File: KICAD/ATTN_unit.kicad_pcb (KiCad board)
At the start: 2 copper layers, 145.5 x 73.5 mm, 5 parts, among them SW1 SW_Push, U1 DM-OLED096-636, U2 HLK-LD2410C, U4 ESP32-DEVKITC-32E

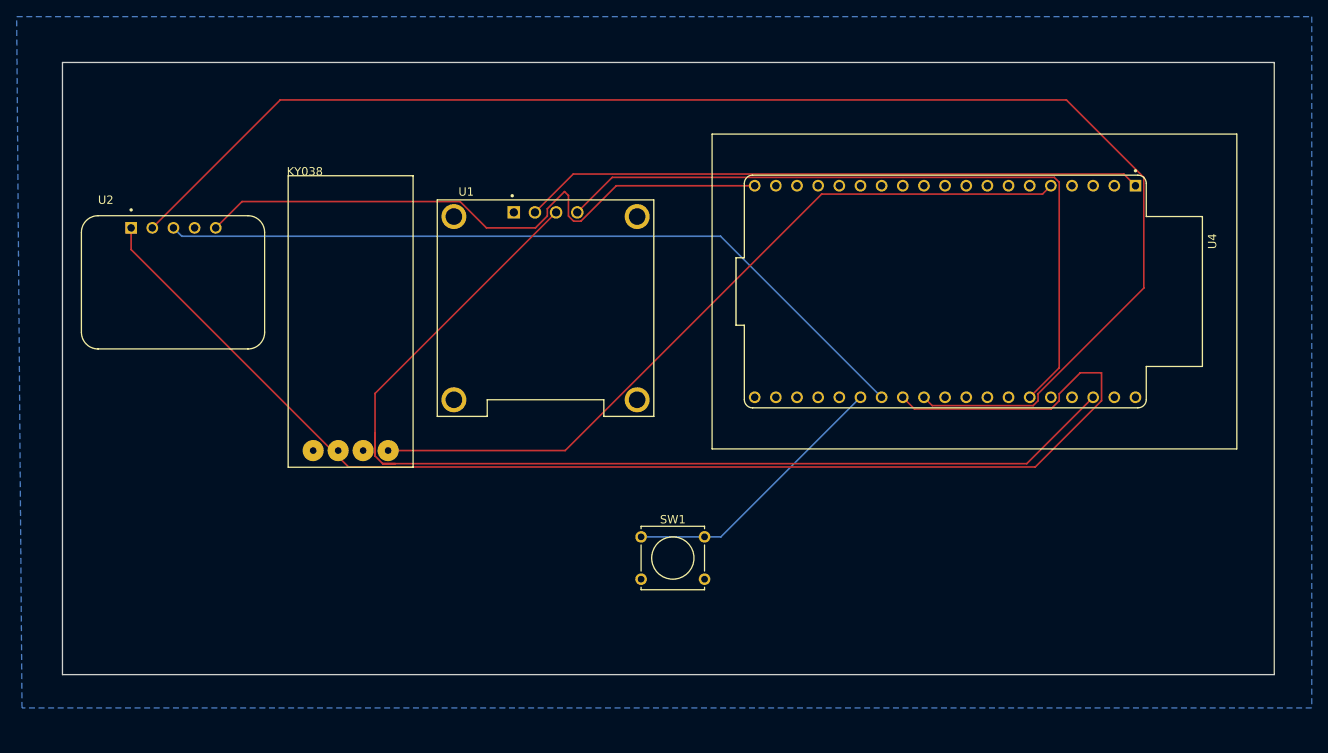
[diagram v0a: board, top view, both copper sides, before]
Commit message: Add files via upload
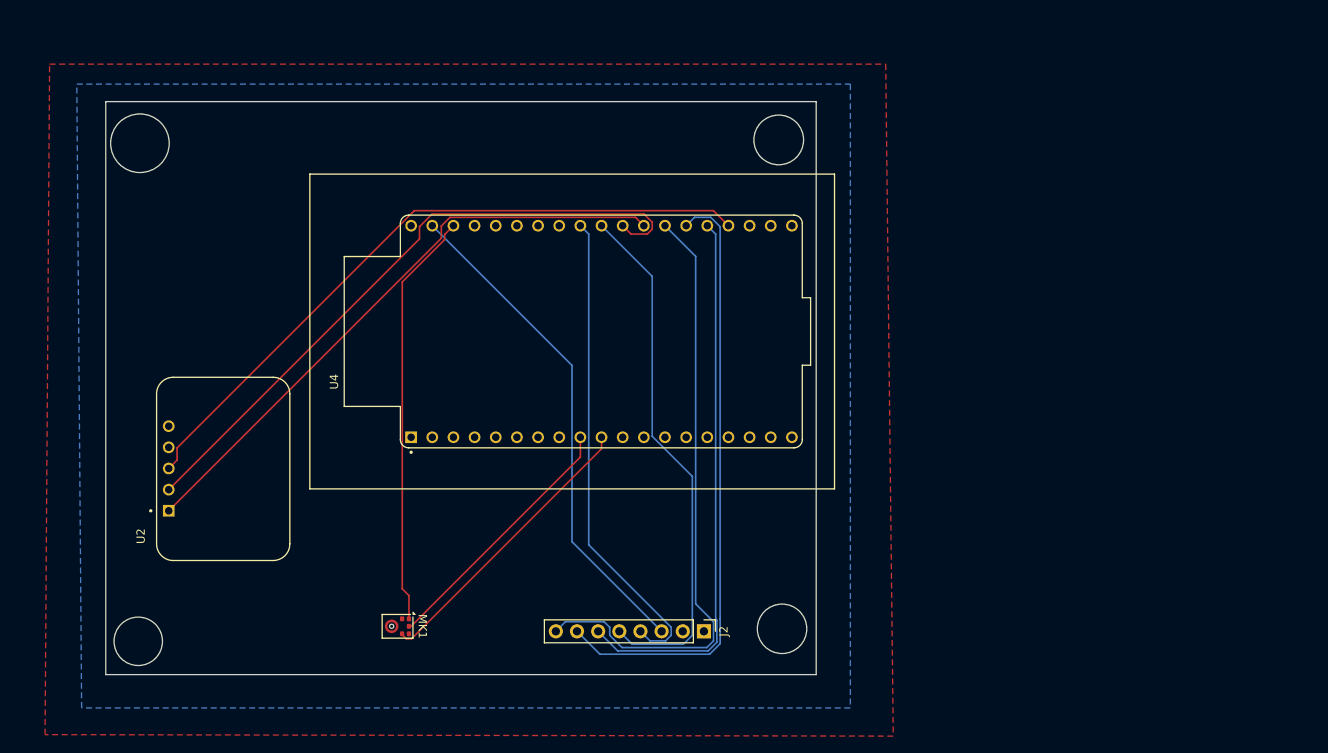
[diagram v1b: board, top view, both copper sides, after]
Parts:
- removed KY038: ~, Custom Boards:KY038
- removed SW1: SW_Push, Button_Switch_THT:SW_Tactile_Straight_KSA0Axx1LFTR
- removed U1: DM-OLED096-636, Custom Boards:OLED Display - 12c - 0.96 inch
- added J2: Screen Connector, Connector_PinHeader_2.54mm:PinHeader_1x08_P2.54mm_Vertical, F.Cu at (152.0, 143.8)
- added MK1: SPH0645LM4H, Sensor_Audio:Knowles_SPH0645LM4H-6_3.5x2.65mm, F.Cu at (115.2, 143.2)
- moved U4 41.6 mm to (139.7, 107.8), turned to 90 degrees
- moved U2 23.2 mm to (94.3, 124.3), turned to 90 degrees
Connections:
- U2 pad 5: Net-(U2-VCC) -> Net-(J2-VCC)
- U4 pad J2_1: Net-(KY038-VCC) -> Net-(J2-VCC)
- U4 pad J2_10: unconnected-(U4-IO26-PadJ2_10) -> Net-(MK1-BCLK)
- U4 pad J2_5: Net-(KY038-AO) -> unconnected-(U4-IO34-PadJ2_5)
- U4 pad J2_9: unconnected-(U4-IO25-PadJ2_9) -> Net-(MK1-DATA)
- U4 pad J3_10: unconnected-(U4-IO5-PadJ3_10) -> Net-(J2-CS)
- U4 pad J3_13: Net-(U2-OUT) -> Net-(J2-BUSY)
- U4 pad J3_15: unconnected-(U4-IO2-PadJ3_15) -> Net-(J2-DC)
- U4 pad J3_16: unconnected-(U4-IO15-PadJ3_16) -> Net-(U2-OUT)
- U4 pad J3_2: unconnected-(U4-IO23-PadJ3_2) -> Net-(J2-DIN)
- U4 pad J3_9: unconnected-(U4-IO18-PadJ3_9) -> Net-(J2-CLK)
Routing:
- net Net-(U2-UART_RX): track 175.7 -> 78.1 mm
- net Net-(KY038-AO): track 92.7 -> 0.00 mm
- net Net-(U2-UART_TX): track 163.3 -> 72.9 mm
- net Net-(U4-IO21): track 87.1 -> 0.00 mm
- net Net-(MK1-WS): track 132.4 -> 50.1 mm
- net Net-(KY038-VCC): track 74.6 -> 0.00 mm
- net Net-(U2-VCC): track 74.3 -> 0.00 mm
- net Net-(J2-BUSY): track 0.00 -> 73.8 mm
- net Net-(J2-DC): track 0.00 -> 66.1 mm
- net Net-(J2-CS): track 0.00 -> 63.6 mm
- net Net-(J2-DIN): track 0.00 -> 60.1 mm
- net Net-(J2-CLK): track 0.00 -> 58.1 mm
- net Net-(J2-RST): track 33.3 -> 73.9 mm
- net Net-(MK1-BCLK): track 0.00 -> 35.1 mm
- net Net-(MK1-DATA): track 0.00 -> 31.4 mm
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- added copper zone on F.Cu, net Net-(J2-VCC)
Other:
- board size 145.5 x 73.5 mm -> 85.3 x 68.8 mm
